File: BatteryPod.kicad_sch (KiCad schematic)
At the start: 26 parts, among them J1 VIN, U1 LM5157RTER

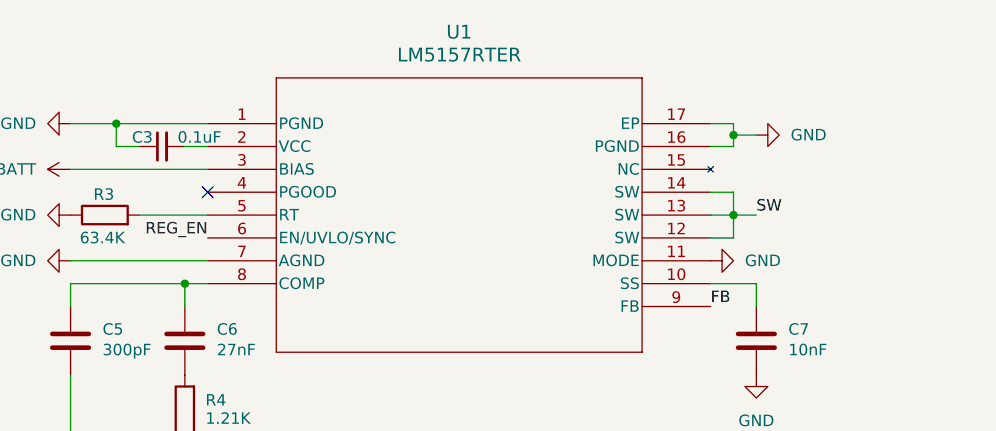
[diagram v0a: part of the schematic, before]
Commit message: patch: final trace cleaups/parameter updates
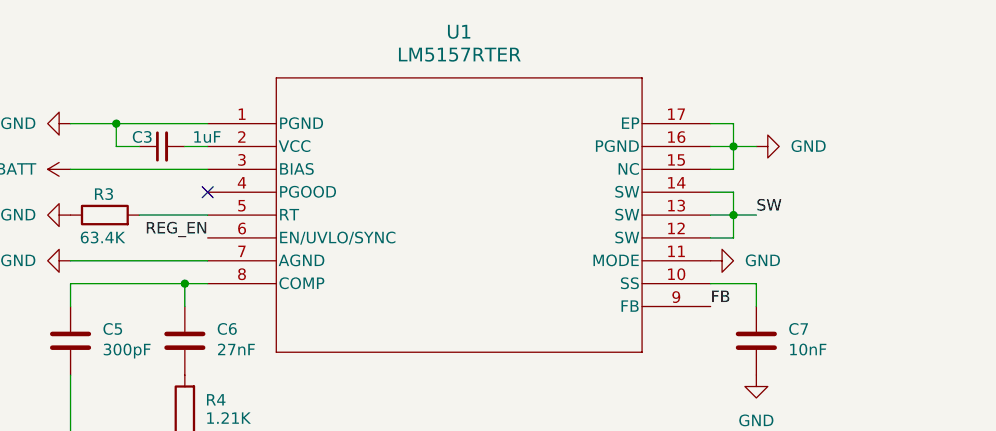
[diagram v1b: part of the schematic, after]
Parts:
- C3: value 0.1uF -> 1uF; Part C597287 -> C342988
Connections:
- net GND: now also U1.15 (NC)
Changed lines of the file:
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@@
+	)
+	(junction
+		(at 163.83 78.74)
+		(diameter 0)
+		(color 0 0 0 0)
 	)
 	(junction
@@
 	)
 	(junction
-		(at 163.83 77.47)
-		(diameter 0)
-		(color 0 0 0 0)
-	)
-	(junction
 		(at 95.25 76.2)
 		(diameter 0)
@@
 	(wire
 		(pts
-			(xy 163.83 76.2) (xy 163.83 77.47)
-		)
-		(stroke
-			(width 0)
-			(type default)
-		)
-	)
-	(wire
-		(pts
 			(xy 102.87 114.3) (xy 96.52 114.3)
 		)
@@
 	(wire
 		(pts
+			(xy 161.29 81.28) (xy 163.83 81.28)
+		)
+		(stroke
+			(width 0)
+			(type default)
+		)
+	)
+	(wire
+		(pts
 			(xy 90.17 81.28) (xy 105.41 81.28)
 		)
@@
 	(wire
 		(pts
-			(xy 166.37 77.47) (xy 163.83 77.47)
+			(xy 166.37 78.74) (xy 163.83 78.74)
 		)
 		(stroke
@@
 	(wire
 		(pts
-			(xy 163.83 78.74) (xy 163.83 77.47)
+			(xy 163.83 76.2) (xy 163.83 78.74)
 		)
 		(stroke
@@
 		(pts
 			(xy 46.99 116.84) (xy 46.99 114.3)
+		)
+		(stroke
+			(width 0)
+			(type default)
+		)
+	)
+	(wire
+		(pts
+			(xy 163.83 81.28) (xy 163.83 78.74)
 		)
 		(stroke
@@
 			)
 		)
-		(property "Part#" ""
-			(at 210.82 119.38 0)
-			(effects
-				(font
-					(size 1.27 1.27)
-				)
-				(hide yes)
-			)
-		)
 		(pin "2"
 		)
@@
 			)
 		)
-		(property "Value" "0.1uF"
+		(property "Value" "1uF"
 			(at 106.934 77.724 90)
 			(effects
@@
 			)
 		)
-		(property "Part" "C597287"
+		(property "Part" "C342988"
 			(at 100.33 78.74 90)
 			(effects
@@
 	(symbol
 		(lib_id "power:GND")
-		(at 166.37 77.47 90)
+		(at 166.37 78.74 90)
 		(unit 1)
 		(exclude_from_sim no)
@@
 		(fields_autoplaced yes)
 		(property "Reference" "#PWR01"
-			(at 172.72 77.47 0)
+			(at 172.72 78.74 0)
 			(effects
 				(font
@@
 		)
 		(property "Value" "GND"
-			(at 170.18 77.4699 90)
+			(at 170.18 78.7399 90)
 			(effects
 				(font
@@
 		)
 		(property "Footprint" ""
-			(at 166.37 77.47 0)
+			(at 166.37 78.74 0)
 			(effects
 				(font
@@
 		)
 		(property "Datasheet" ""
-			(at 166.37 77.47 0)
+			(at 166.37 78.74 0)
 			(effects
 				(font
@@
 		)
 		(property "Description" "Power symbol creates a global label with name \"GND\" , ground"
-			(at 166.37 77.47 0)
-			(effects
-				(font
+			(at 166.37 78.74 0)
+			(effects
+				(font
